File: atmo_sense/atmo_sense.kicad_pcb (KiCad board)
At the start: 4 copper layers, 57 x 59 mm, 54 parts, among them J1 Conn_01x04_Pin, J2 USB-C, J3 TB007-508-02BE, J4 Conn_02x05_Top_Bottom, J5 Conn_01x04_Pin, SW1 SW_Push, SW2 SW_Push, SW3 SW_Push, U1 USBLC6-2SC6, U2 ESP32-C3FH4, U3 BME680, U4 LM1117LD-3.3, Y1 ECS-400-10-36B2-CKM-TR, Y2 Crystal

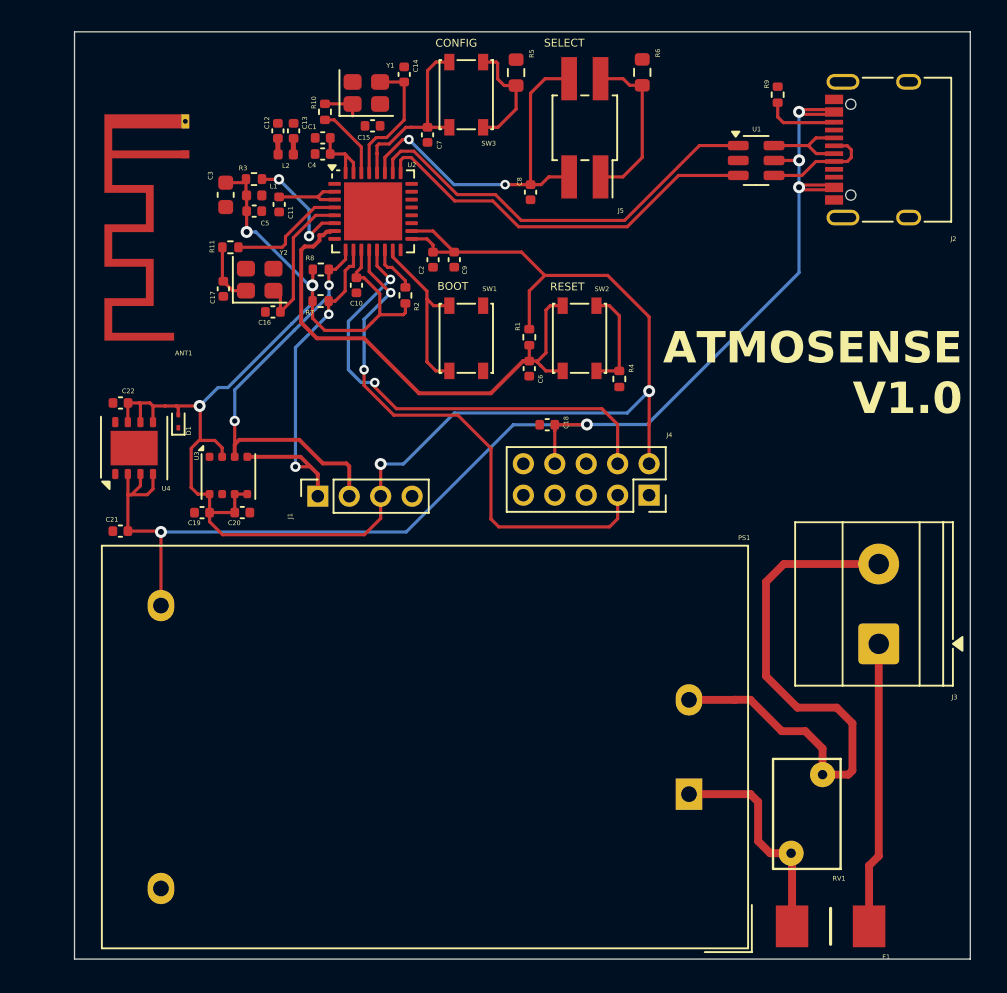
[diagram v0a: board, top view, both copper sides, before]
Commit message: PCB design
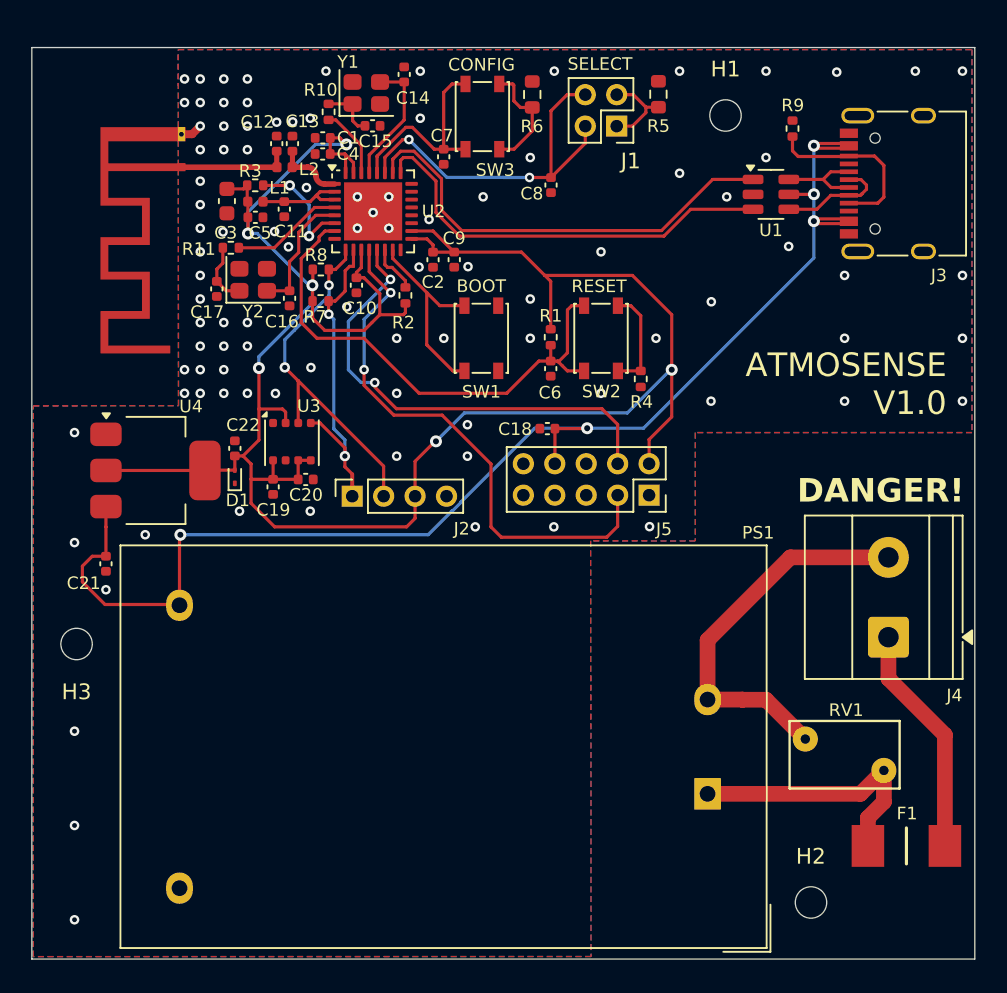
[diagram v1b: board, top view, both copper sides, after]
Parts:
- added H1: MountingHole, MountingHole:MountingHole_2mm, F.Cu at (140.4, 56.3)
- added H2: MountingHole, MountingHole:MountingHole_2mm, F.Cu at (145.9, 106.4)
- added H3: MountingHole, MountingHole:MountingHole_2mm, F.Cu at (99.1, 90.0)
- J1: renamed from J5; footprint Connector_PinSocket_2.00mm:PinSocket_2x02_P2.00mm_Vertical_SMD -> Connector_PinSocket_2.00mm:PinSocket_2x02_P2.00mm_Vertical
- U4: value LM1117LD-3.3 -> AMS1117-3.3; footprint Package_SON:WSON-8-1EP_4x4mm_P0.8mm_EP2.2x3mm -> Package_TO_SOT_SMD:SOT-223-3_TabPin2
- moved RV1 7.91 mm to (150.5, 98.0), turned to 180 degrees
- moved C22 7.83 mm to (109.2, 77.5), turned to 90 degrees
- moved F1 7.03 mm to (151.9, 102.8)
- moved D1 5.04 mm to (109.2, 79.3)
- moved C19 4.81 mm to (111.6, 80.0), turned to -90 degrees
- moved U3 4.58 mm to (112.8, 77.1)
- moved C20 4.55 mm to (113.7, 79.5)
- moved R9 2.35 mm to (144.7, 57.2)
- moved U1 2.35 mm to (143.3, 61.3)
- moved J3 2.35 mm to (151.9, 60.7)
- moved C21 2.27 mm to (101.0, 84.8), turned to -90 degrees
- moved J2 2.19 mm to (116.7, 80.5)
- moved J1 2.03 mm to (133.5, 57.0)
- moved U4 1.97 mm to (104.1, 78.9), turned to 0 degrees
- moved R6 1.73 mm to (128.1, 55.0)
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- renumbered J1 to J2, J2 to J3, J3 to J4, J4 to J5, R6 to R5, R5 to R6
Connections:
- net /CHIP_EN renamed /RESET
- U4 pad 2: +5V -> +3.3V
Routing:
- net Net-(J4-Pin_2): track 36.8 -> 24.7 mm
- net +3.3V: track 132.7 -> 144.7 mm, vias 5 -> 6
- net /CC1: track 4.66 -> 11.5 mm
- net /RF_ANT: track 1.03 -> 7.11 mm
- net Net-(J1-Pin_1): track 10.6 -> 5.55 mm
- net /SDA: track 26.4 -> 22.8 mm
- net Net-(J4-Pin_1): track 18.2 -> 14.8 mm
- net /LNA_IN: track 1.03 -> 4.32 mm
- net /SCL: track 23.7 -> 20.7 mm
- net Net-(PS1-AC/L): track 14.2 -> 17.1 mm
- net Net-(C15-Pad1): track 2.53 -> 4.30 mm
- net /USB_DP: track 26.9 -> 28.6 mm
- net /USB_DN: track 25.5 -> 27.2 mm
- net /XTAL_32_N: track 9.81 -> 8.13 mm
- net /GPI09: track 11.3 -> 12.8 mm
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- added copper zone on B.Cu, net GND
- added copper zone on F.Cu, net GND
- added copper zone on In1.Cu, net GND
- added copper zone on In2.Cu, net GND
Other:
- board size 57 x 59 mm -> 60 x 58 mm
- board text added: "DANGER!"
